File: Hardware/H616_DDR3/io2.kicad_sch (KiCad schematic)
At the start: 16 parts, among them U1 H616, Y1 24MHz

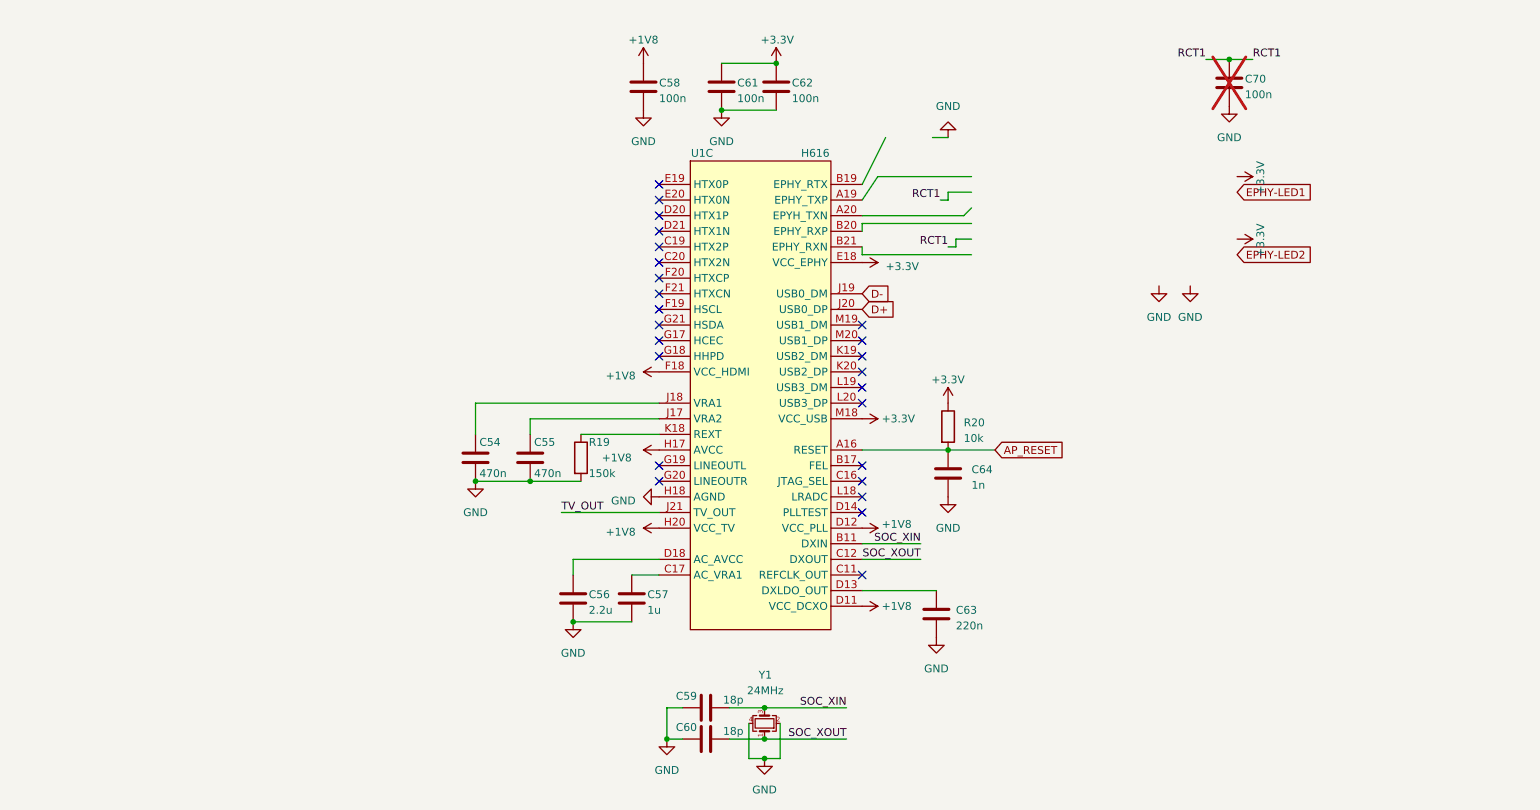
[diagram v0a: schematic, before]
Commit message: radio+hdr
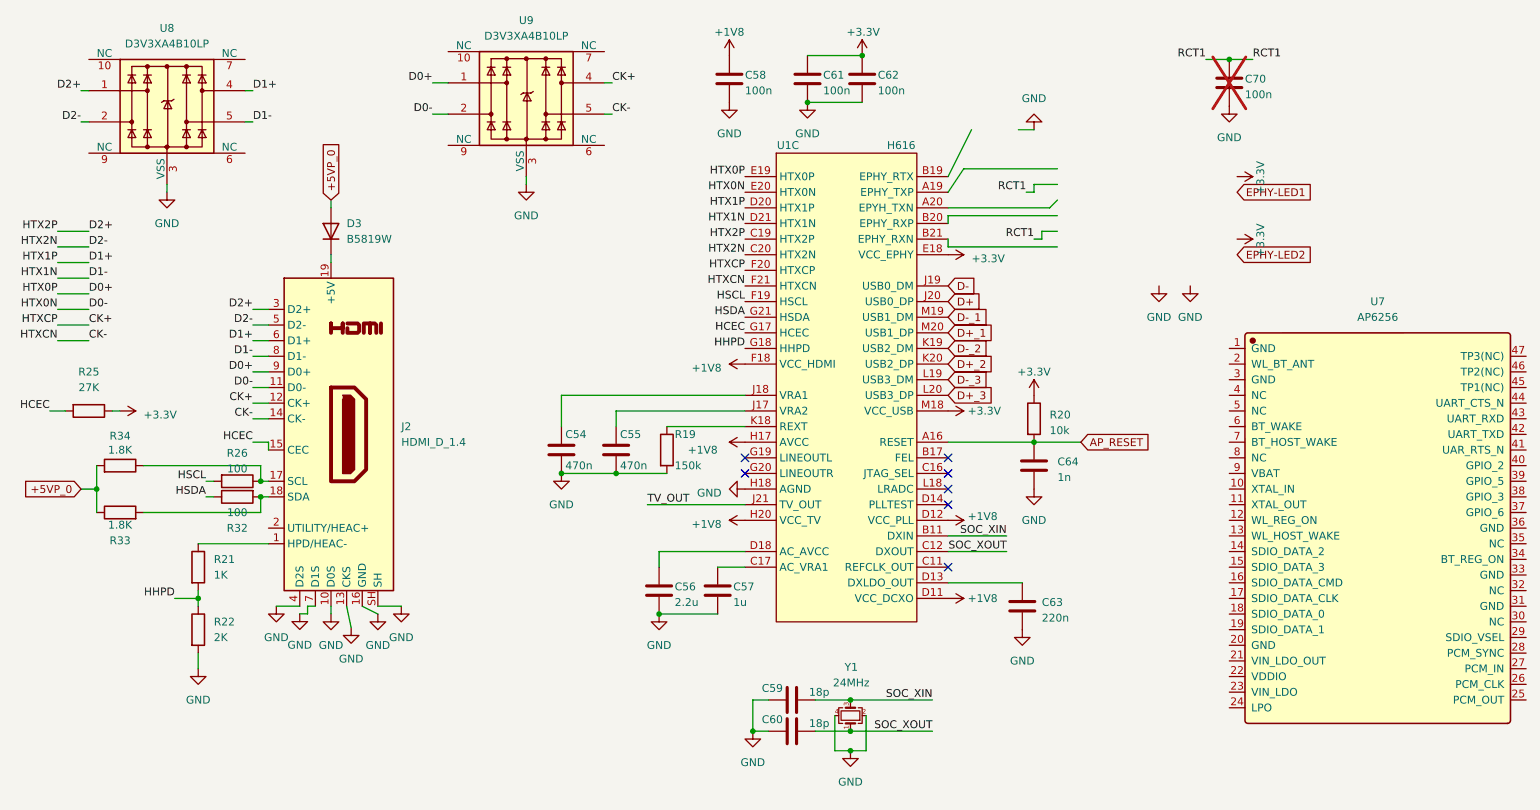
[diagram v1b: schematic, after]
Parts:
- added D3: B5819W, Diode_SMD:D_SOD-123, symbol Diode:1N4148W
- added J2: HDMI_D_1.4, Connector_Video:HDMI_Micro-D_Molex_46765-1xxx, symbol Connector:HDMI_D_1.4
- added R21: 1K, Resistor_SMD:R_0402_1005Metric, symbol Device:R
- added R22: 2K, Resistor_SMD:R_0402_1005Metric, symbol Device:R
- added R25: 27K, Resistor_SMD:R_0402_1005Metric, symbol Device:R
- added R26, R32: 100, Resistor_SMD:R_0402_1005Metric, symbol Device:R
- added R33, R34: 1.8K, Resistor_SMD:R_0402_1005Metric, symbol Device:R
- added U7: AP6256, bodya:AP6255, symbol JLCImport:AP6256
- added U8, U9: D3V3XA4B10LP, Package_DFN_QFN:Diodes_UDFN-10_1x2.5mm_P0.5mm, symbol Power_Protection:D3V3XA4B10LP
- C54, C55, C56, C57, C58, C59, C60, C61, C62, C63, C64, C70: footprint Capacitor_SMD:C_0402_1005Metric_Pad0.74x0.62mm_HandSolder -> Capacitor_SMD:C_0402_1005Metric
- R19, R20: footprint Resistor_SMD:R_0402_1005Metric_Pad0.72x0.64mm_HandSolder -> Resistor_SMD:R_0402_1005Metric
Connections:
- net +3.3V: now also R25.1
- net GND: now also J2.10 (D0S), J2.13 (CKS), J2.16 (GND), J2.4 (D2S), J2.7 (D1S), J2.SH, R22.2, U8.3 (VSS), U8.8 (VSS), U9.3 (VSS), U9.8 (VSS)
- net D2+: now reaches U1.C19 (HTX2P)
- net D2+: now also J2.3 (D2+), U8.1
- net D2-: now reaches U1.C20 (HTX2N)
- net D2-: now also J2.5 (D2-), U8.2
- net D1+: now reaches U1.D20 (HTX1P)
- net D1+: now also J2.6 (D1+), U8.4
- net D1-: now reaches U1.D21 (HTX1N)
- net D1-: now also J2.8 (D1-), U8.5
- net D0+: now reaches U1.E19 (HTX0P)
- net D0+: now also J2.9 (D0+), U9.1
- net D0-: now reaches U1.E20 (HTX0N)
- net D0-: now also J2.11 (D0-), U9.2
- net HSCL: now reaches U1.F19 (HSCL)
- net HSCL: now also R26.2
- net CK+: now reaches U1.F20 (HTXCP)
- net CK+: now also J2.12 (CK+), U9.4
- net CK-: now reaches U1.F21 (HTXCN)
- net CK-: now also J2.14 (CK-), U9.5
- net HCEC: now reaches U1.G17 (HCEC)
- net HCEC: now also J2.15 (CEC), R25.2
- net HHPD: now reaches U1.G18 (HHPD)
- net HHPD: now also R21.2, R22.1
- net HSDA: now reaches U1.G21 (HSDA)
- net HSDA: now also R32.1
- net D-_2: now reaches U1.K19 (USB2_DM)
- net D+_2: now reaches U1.K20 (USB2_DP)
- net D-_3: now reaches U1.L19 (USB3_DM)
- net D+_3: now reaches U1.L20 (USB3_DP)
- net D-_1: now reaches U1.M19 (USB1_DM)
- net D+_1: now reaches U1.M20 (USB1_DP)
- new net: J2.17 (SCL), R26.1, R34.1
- new net: J2.18 (SDA), R32.2, R33.2
- new net: J2.1 (HPD/HEAC-), R21.1
- new net: D3.1 (K), J2.19 (+5V)
- new net +5VP_0: D3.2 (A), R33.1, R34.2
- no-connect marks 25 -> 7
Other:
- moved on the sheet: C54, C55, C56, C57, C58, C59, C60, C61, C62, C63, C64, R19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
